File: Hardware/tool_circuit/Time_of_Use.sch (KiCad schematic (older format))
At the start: 2 parts

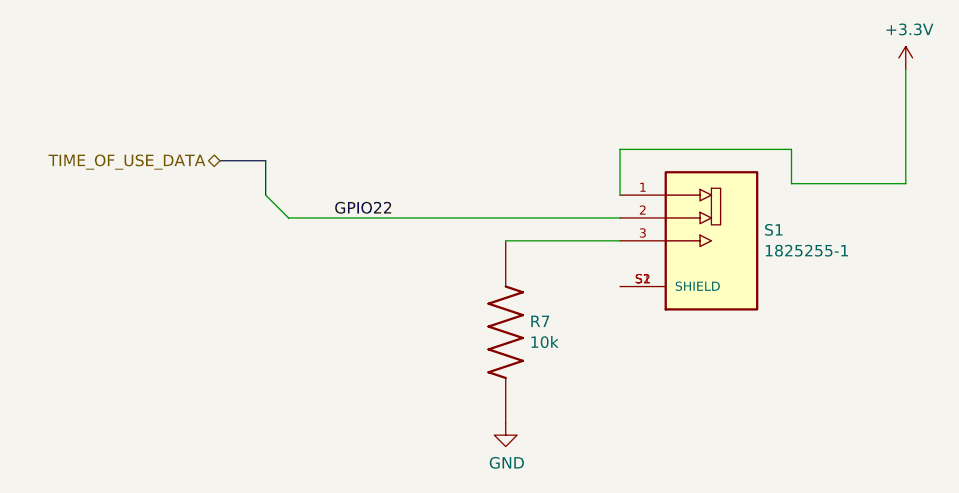
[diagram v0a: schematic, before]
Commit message: PCB changes
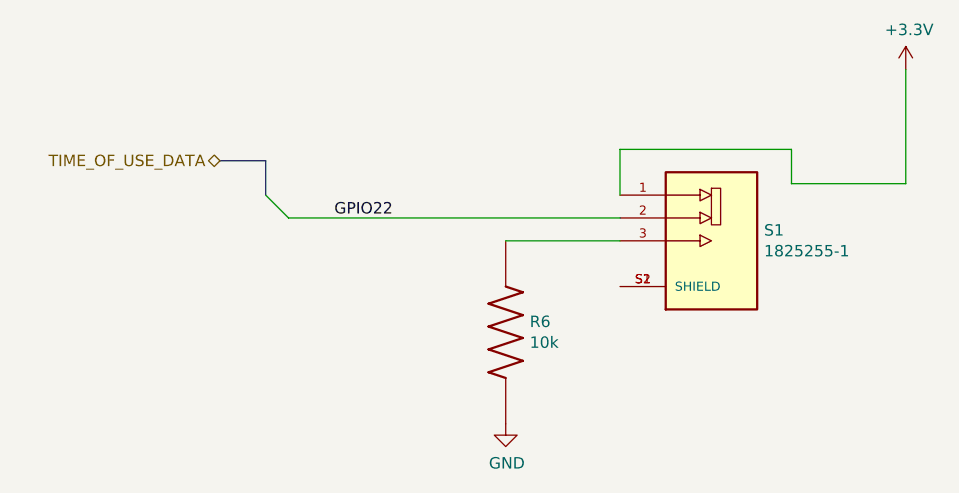
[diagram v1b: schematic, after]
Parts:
- R6: renamed from R7; footprint RESC3115X60N -> RNCP1206FTD10K0:RESC3115X60N
- S1: footprint SW_1825255-1 -> 1825255-1:SW_1825255-1
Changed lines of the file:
@@
 F 0 "S1" H 6030 4296 50  0000 L CNN
 F 1 "1825255-1" H 6030 4205 50  0000 L CNN
-F 2 "SW_1825255-1" H 5800 4250 50  0001 L BNN
+F 2 "1825255-1:SW_1825255-1" H 5800 4250 50  0001 L BNN
 F 3 "" H 5800 4250 50  0001 L BNN
 F 4 "1825255-1" H 5800 4250 50  0001 L BNN "Comment"
@@
 	4900 4250 5400 4250
 $Comp
-L RNCP1206FTD10K0:RNCP1206FTD10K0 R7
+L RNCP1206FTD10K0:RNCP1206FTD10K0 R6
 U 1 1 617867AC
 P 4900 4650
-F 0 "R7" V 4854 4755 50  0000 L CNN
+F 0 "R6" V 4854 4755 50  0000 L CNN
 F 1 "10k" V 4945 4755 50  0000 L CNN
-F 2 "RESC3115X60N" H 4900 4650 50  0001 L BNN
+F 2 "RNCP1206FTD10K0:RESC3115X60N" H 4900 4650 50  0001 L BNN
 F 3 "" H 4900 4650 50  0001 L BNN
 	1    4900 4650
